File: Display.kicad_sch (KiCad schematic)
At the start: 7 parts, among them U2 HPDL1414, U3 HPDL1414, U4 HPDL1414, U7 74AHC595

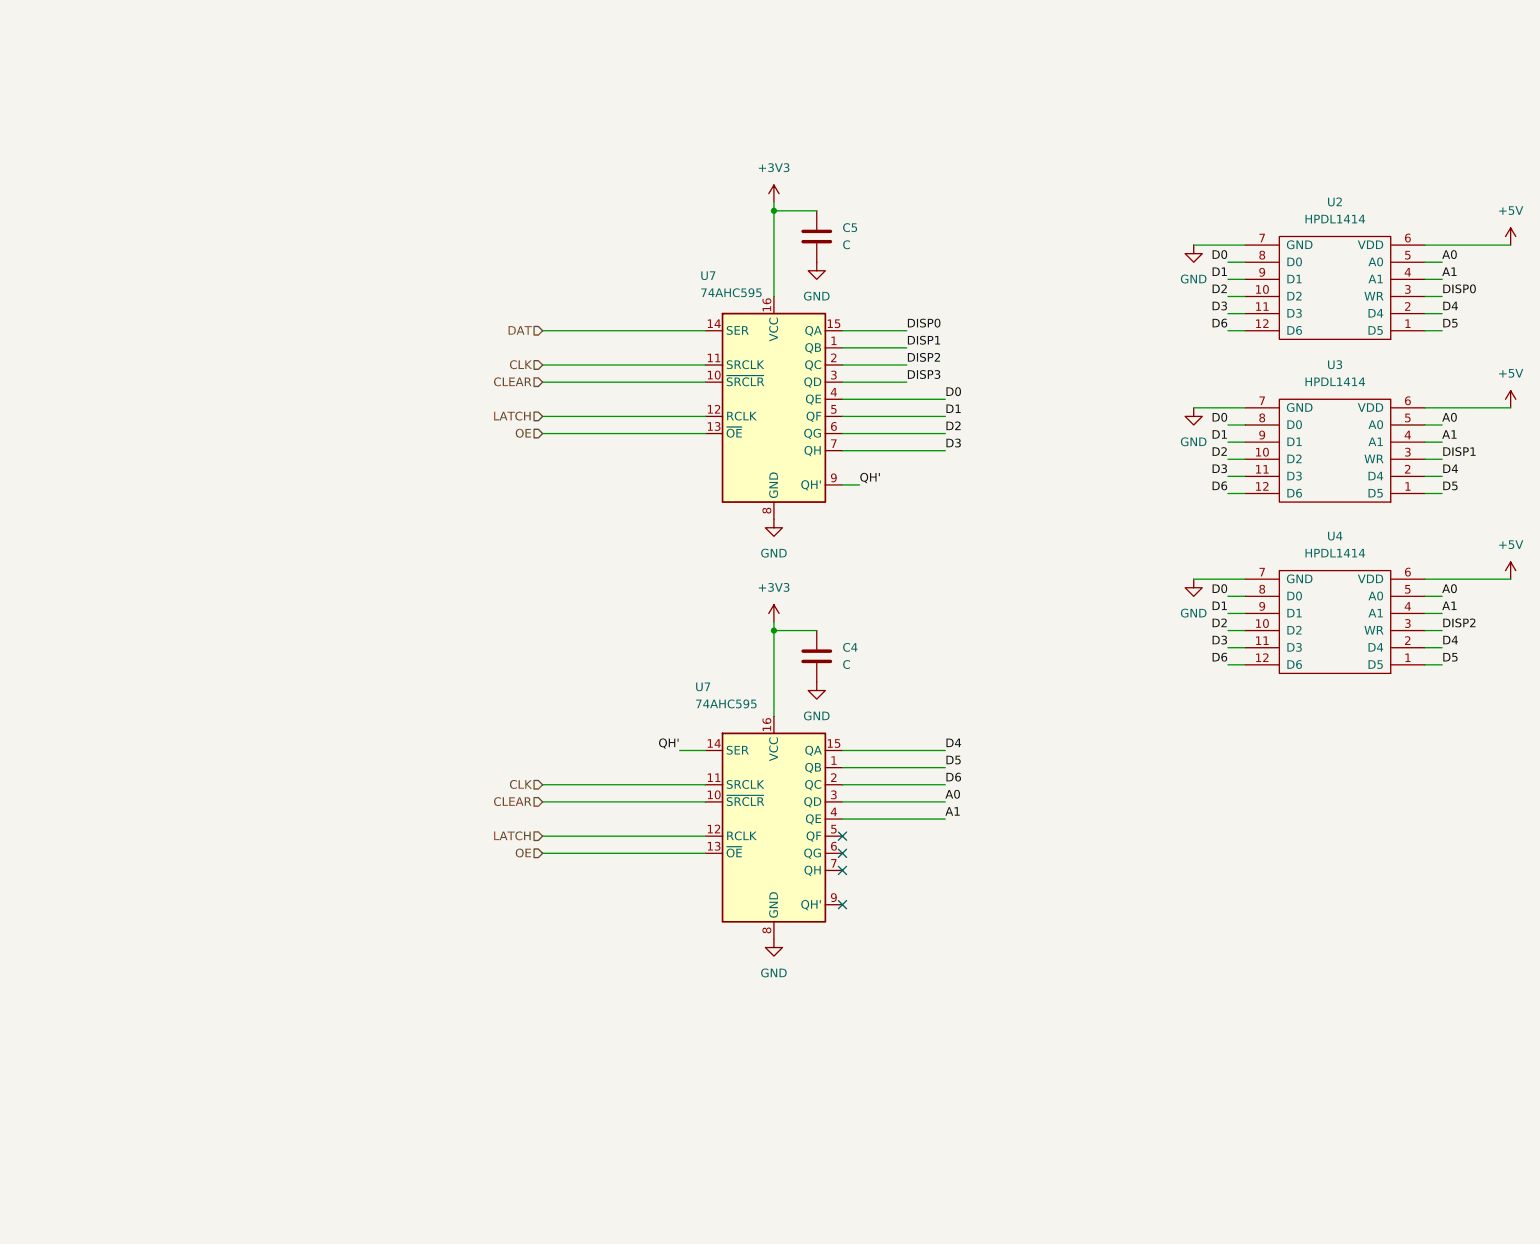
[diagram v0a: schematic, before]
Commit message: Update
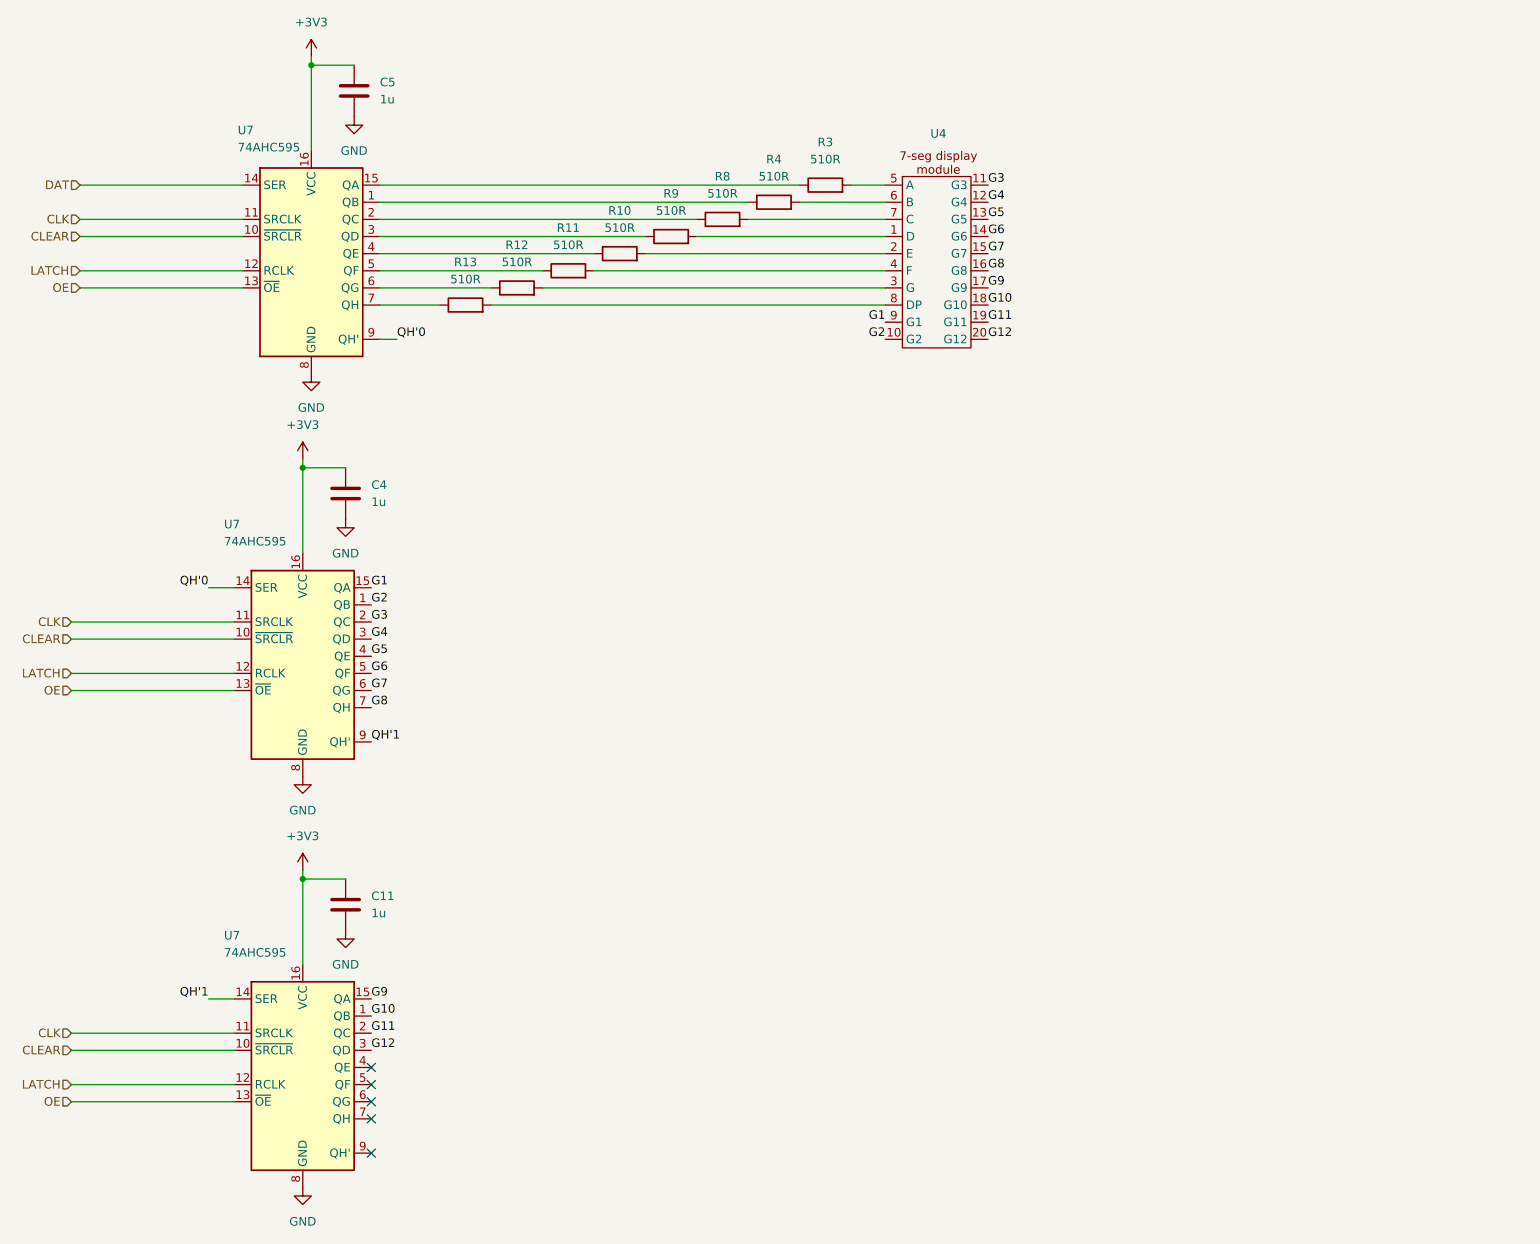
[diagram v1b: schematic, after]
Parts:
- removed U2, U3, U4: HPDL1414, DL1414:HPDLDL-1414, symbol DL1414:HPDL1414
- added C11: 1u, symbol Device:C
- added R10, R11, R12, R13, R3, R4, R8, R9: 510R, symbol Device:R
- added U4: ~, footprints:display, symbol project parts:display
- added U7: 74AHC595, symbol 74xx:74AHC595
- C4, C5: value C -> 1u
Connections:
- net +3V3: now also C11.1, U7.16 (VCC)
- net CLEAR: now also U7.10 (~{SRCLR})
- net CLK: now also U7.11 (SRCLK)
- net GND: now also C11.2, U7.8 (GND)
- net LATCH: now also U7.12 (RCLK)
- net OE: now also U7.13 (~{OE})
- net G6: now reaches U7.5 (QF)
- net G6: now also U4.14 (G6)
- net G7: now reaches U7.6 (QG)
- net G7: now also U4.15 (G7)
- net G8: now reaches U7.7 (QH)
- net G8: now also U4.16 (G8)
- net QH'1: now reaches U7.9 (QH')
- net QH'1: now also U7.14 (SER)
- net A0 renamed G4
- net G4: now also U4.12 (G4)
- net A1 renamed G5
- net G5: now also U4.13 (G5)
- net D0: no longer names the net of U7.4 (QE)
- net D0: now also R10.1
- net D1: no longer names the net of U7.5 (QF)
- net D1: now also R11.1
- net D2: no longer names the net of U7.6 (QG)
- net D2: now also R12.1
- net D3: no longer names the net of U7.7 (QH)
- net D3: now also R13.1
- net D4 renamed G1
- net G1: now also U4.9 (G1)
- net D5 renamed G2
- net G2: now also U4.10 (G2)
- net D6 renamed G3
- net G3: now also U4.11 (G3)
- net DISP0: no longer names the net of U7.15 (QA)
- net DISP0: now also R3.1
- net DISP1: no longer names the net of U7.1 (QB)
- net DISP1: now also R4.1
- net DISP2: no longer names the net of U7.2 (QC)
- net DISP2: now also R8.1
- net DISP3: no longer names the net of U7.3 (QD)
- net DISP3: now also R9.1
- net QH' renamed QH'0
- new net: R10.2, U4.2 (E)
- new net: R12.2, U4.3 (G)
- new net: R8.2, U4.7 (C)
- new net: R11.2, U4.4 (F)
- new net: R13.2, U4.8 (DP)
- new net: R9.2, U4.1 (D)
- new net: R3.2, U4.5 (A)
- new net: R4.2, U4.6 (B)
- new net G10: U4.18 (G10), U7.1 (QB)
- new net G11: U4.19 (G11), U7.2 (QC)
- new net G12: U4.20 (G12), U7.3 (QD)
- new net G9: U4.17 (G9), U7.15 (QA)
- no-connect marks 4 -> 5
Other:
- moved on the sheet: C4, C5, U7
